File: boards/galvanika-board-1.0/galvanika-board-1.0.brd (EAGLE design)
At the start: 100 x 80 mm, 95 parts, among them IC1 LM358D, IC2 7805DT, IC3 74HCT595D, IC4 74HCT595D, IC5 74HCT595D, IC6 ATMEGA48/88/168-PU, Q1 20MHz

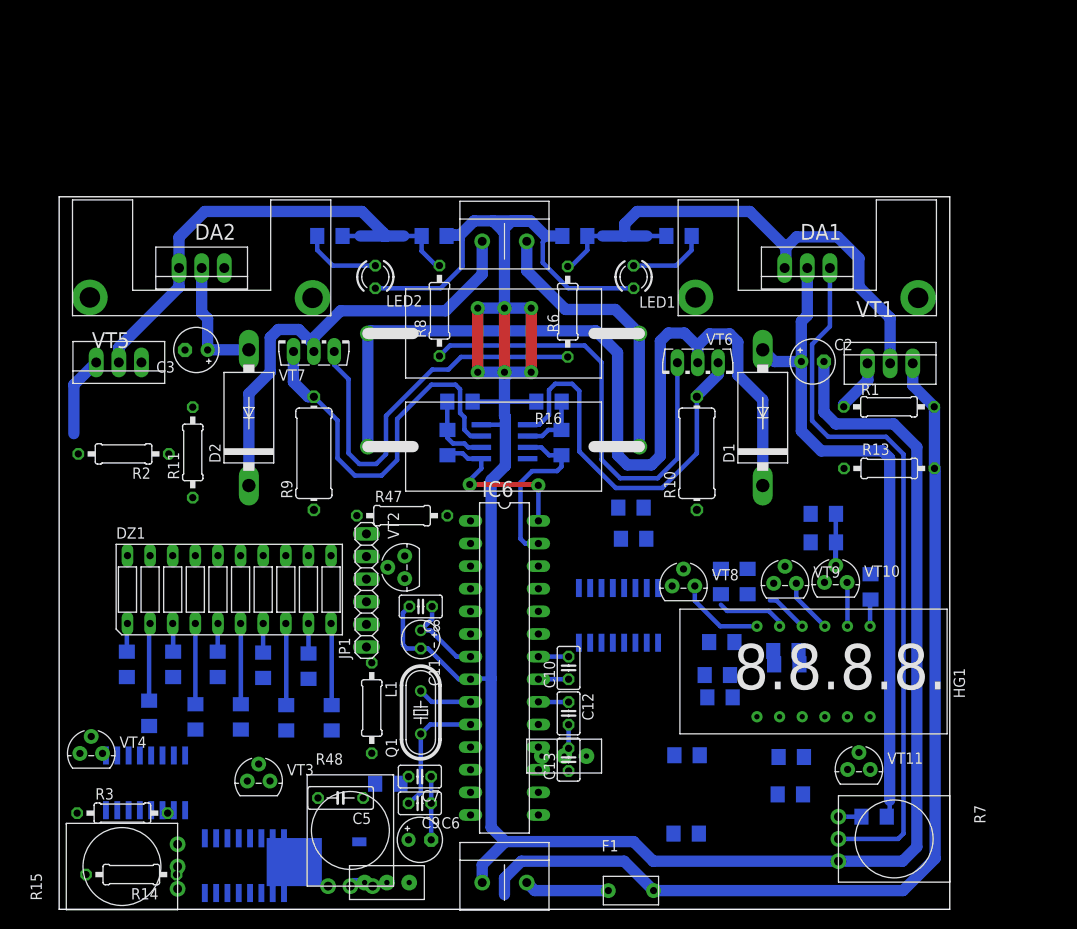
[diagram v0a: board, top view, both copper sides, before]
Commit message: 'board'
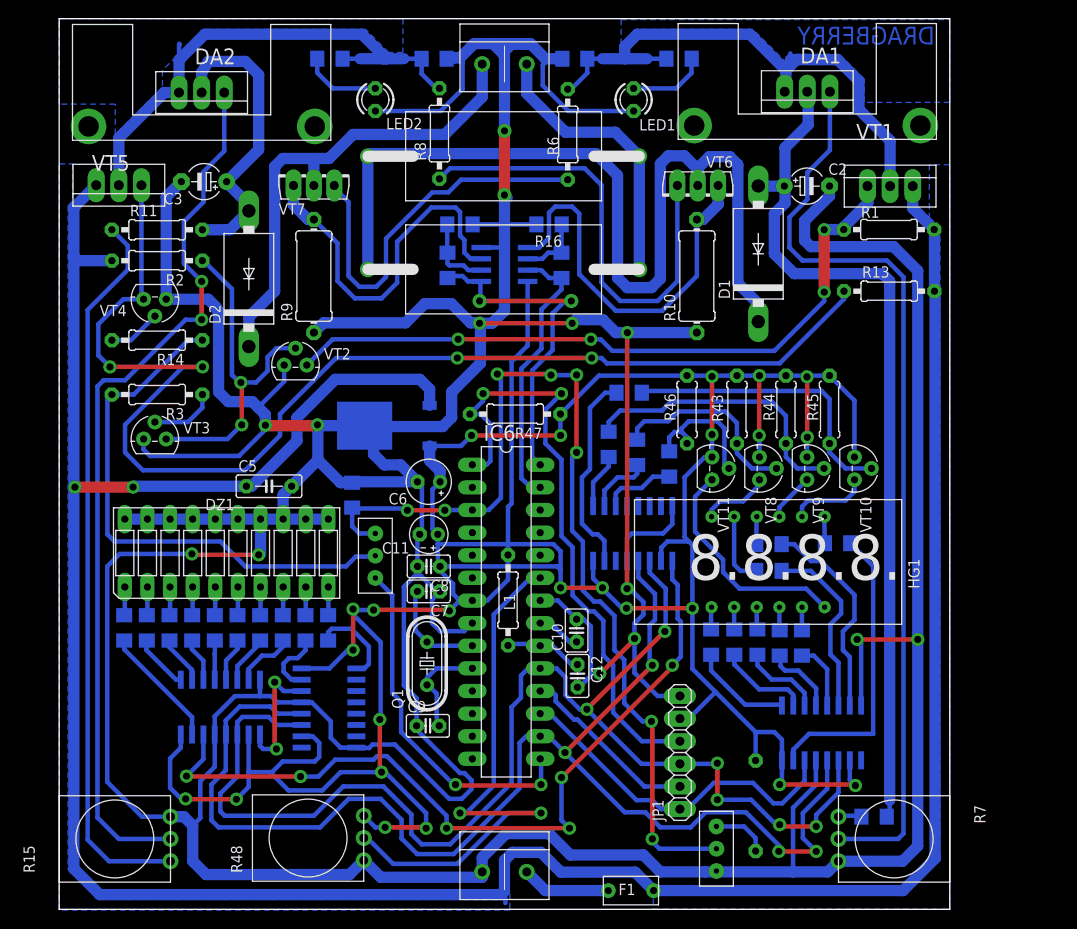
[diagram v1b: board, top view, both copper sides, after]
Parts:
- added IC7: 74HC595D, 74xx-eu:SO16
- C13: device rcl:C025-025X050 -> rcl:C1206
- C2, C3: device rcl:E2,5-5 -> rcl:E5-4
- R43, R44, R45, R46: device rcl:R1206 -> rcl:0207/7
- R49: device rcl:R1206 -> rcl:0207/10
- moved IC4 61.4 mm to (64.4, 42.2)
- moved R14 60.1 mm to (11.0, 63.9)
- moved VT4 51.5 mm to (10.7, 68.5), turned to 180 degrees
- moved IC2 49.6 mm to (36.8, 54.3)
- moved R46 47.6 mm to (70.5, 56.1), flipped to the top, turned to 90 degrees
- moved R3 47.2 mm to (11.0, 57.8), turned to 180 degrees
- moved R44 43.2 mm to (81.6, 56.1), flipped to the top, turned to 90 degrees
- moved R49 41.4 mm to (78.2, 11.6), turned to 90 degrees
- moved C6 40.2 mm to (41.5, 48.0), turned to 180 degrees
- moved VT3 40.1 mm to (10.8, 52.8)
- moved JP1 39.6 mm to (69.7, 17.6)
- moved R43 39.5 mm to (76.1, 56.1), flipped to the top, turned to 90 degrees
- moved C13 38.4 mm to (32.9, 46.5), flipped to the bottom
- moved VT11 37.6 mm to (73.3, 49.5), turned to 270 degrees
- moved SA1 36.7 mm to (35.5, 39.7), turned to 90 degrees
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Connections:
- net N$87 renamed PWM
- removed net N$50 (its old number): IC5.3, R28.2
- removed net N$65: IC3.5, R36.1
- removed net N$66: IC3.6, R37.1
- removed net N$67: IC3.7, R38.1
- removed net N$68: IC3.14, IC6.17, JP1.4
- removed net N$86: IC3.12, IC4.12, IC5.12, IC6.16
- removed net N$89: C13.1, IC6.14, SA1.1$S, SA2.1$P
- new net CLOCK: IC3.11, IC4.11, IC5.11, IC6.19, IC7.11, JP1.3
- new net DATA: IC3.14, IC6.17, JP1.1
- new net LATCH: IC3.12, IC4.12, IC5.12, IC6.16, IC7.12
- new net N$29: IC5.1, R22.1
- new net N$41: DZ1.7, R27.1
- new net N$55: IC3.6, R31.1
- new net PWM-CTRL: C13.1, IC6.3, SA1.1$S, SA2.1$P
- net +19V: no longer R49.2
- net GND: now also IC7.13, IC7.8, R15.3, VT2.3, VT3.3, VT4.3; no longer R15.1
- net N$16: now also IC3.3, R38.1; no longer IC3.2, R33.1
- net N$17: now also IC3.2, R34.1; no longer IC3.15, R31.1
- net N$21: now also R15.1; no longer R15.3
- net N$24: now also JP1.2; no longer JP1.3
- net N$30: now also R22.2; no longer R23.1
- net N$31: now also IC5.2, R23.2; no longer DZ1.3, R25.1
- net N$32: now also DZ1.3, R23.1; no longer DZ1.4, R27.1
- net N$33: now also DZ1.4, R24.1; no longer DZ1.5, R29.1
- net N$34: now also IC5.3, R24.2; no longer IC5.5, R30.1
- net N$35: now also IC3.5, R37.1; no longer IC3.11, IC4.11, IC5.11, IC6.19, JP1.2
- net N$36: now also IC5.4, R25.2; no longer IC4.4, R21.1
- net N$37: now also DZ1.5, R25.1; no longer DZ1.6, R22.2
- net N$38: now also IC5.5, R26.2; no longer DZ1.7, R24.1
- net N$39: now also DZ1.6; no longer DZ1.8
- net N$4: now also IC5.15, R21.1; no longer VT2.3, VT3.3, VT4.3
- net N$40: now also IC5.6, R27.2; no longer DZ1.9, R28.1
- net N$42: now also IC5.7, R28.2; no longer IC4.5, R22.1
- net N$43: now also DZ1.8, R28.1; no longer IC4.6, R23.2
- net N$44: now also IC3.7, R36.1; no longer IC4.7, R24.2
- net N$47: now also IC5.9, IC7.14; no longer IC5.15, R25.2
- net N$48: now also IC7.15, R29.2; no longer IC5.1, R26.2
- net N$49: now also IC7.1, R30.1; no longer IC5.2, R27.2
- net N$51: now also DZ1.9, R29.1; no longer IC5.4, R29.2
- net N$61: now also IC3.15; no longer IC3.1
- net N$64: now also IC3.1; no longer IC3.4
- net N$7: now also IC3.4, R33.1; no longer IC3.3, R34.1
- net N$73: now also R41.2; no longer R39.2
- net N$75: now also R39.2; no longer R41.2
- net N$85: now also JP1.4; no longer JP1.1
- net VCC: now also IC7.10, IC7.16, R49.2
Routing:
- net GND: track 303.7 -> 745.0 mm, vias 6 -> 14
- net VCC: track 10.0 -> 378.4 mm, vias 0 -> 24
- net +19V: track 119.6 -> 313.9 mm, vias 0 -> 2
- net LATCH: track 0.00 -> 149.2 mm, vias 0 -> 4
- net CLOCK: track 0.00 -> 146.3 mm, vias 0 -> 6
- net N$20: track 0.00 -> 141.7 mm, vias 0 -> 4
- net PWM-CTRL: track 0.00 -> 110.3 mm, vias 0 -> 8
- net N$23: track 0.00 -> 100.6 mm, vias 0 -> 2
- net N$45: track 0.00 -> 90.0 mm, vias 0 -> 6
- net N$21: track 0.00 -> 81.4 mm
- net N$1: track 6.08 -> 78.4 mm, vias 0 -> 4
- net N$85: track 0.00 -> 69.7 mm, vias 0 -> 2
- net N$88: track 0.00 -> 63.8 mm, vias 0 -> 2
- net N$25: track 0.00 -> 61.2 mm
- net PWM: track 0.00 -> 39.8 mm, vias 0 -> 2
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- added copper zone on layer 16, net +19V
- added copper zone on layer 16, net VI-LEFT
- added copper zone on layer 16, net VI-RIGHT
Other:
- board size 100 x 80 mm -> 100 x 100 mm
- board text added: "DRAGBERRY"
